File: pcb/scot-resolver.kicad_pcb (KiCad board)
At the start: 2 copper layers, 146 parts, among them IC1 AD8692ARMZ, IC10 AD2S1210, IC2 AD8397ARZ, IC3 AD8692ARMZ, IC4 TSR1, IC5 AD8692ARMZ, IC6 AD8692ARMZ, IC7 AD8692ARMZ, IC8 MCP2562, IC9 STM32F0xxKxTx, J1 Conn_01x02_Female, J2 Conn_01x02_Female, J3 Conn_01x02_Female, J4 Conn_01x03_Female, J5 Conn_01x03_Female, J6 Conn_01x03_Female, J7 CONN_01x03, P1 SWD, U1 MCP1703A-5002_SOT223, U2 LT1762, U3 MCP1703A-5002_SOT223, U4 MCP1703A-5002_SOT223, U5 MCP1703A-3302_SOT223, Y1 Crystal_GND24, Y2 Crystal

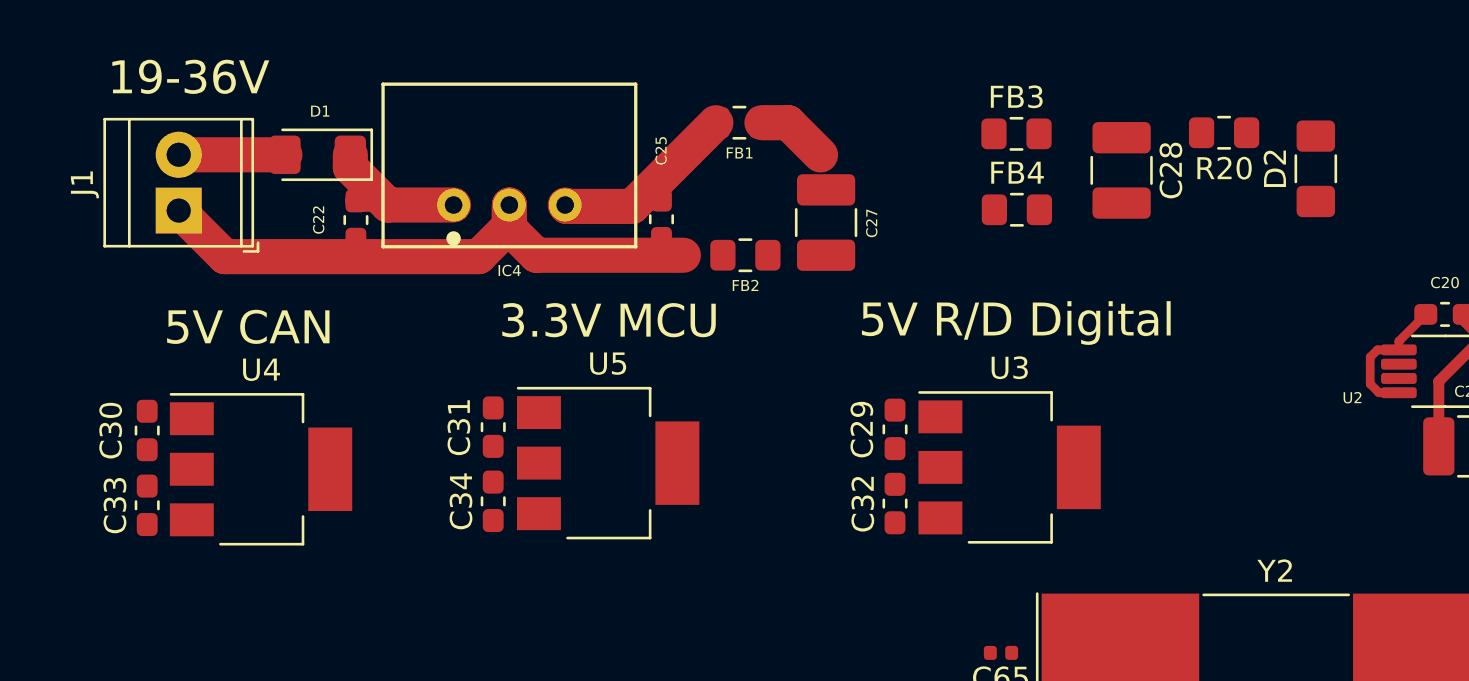
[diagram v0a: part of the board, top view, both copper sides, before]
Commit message: WIP.
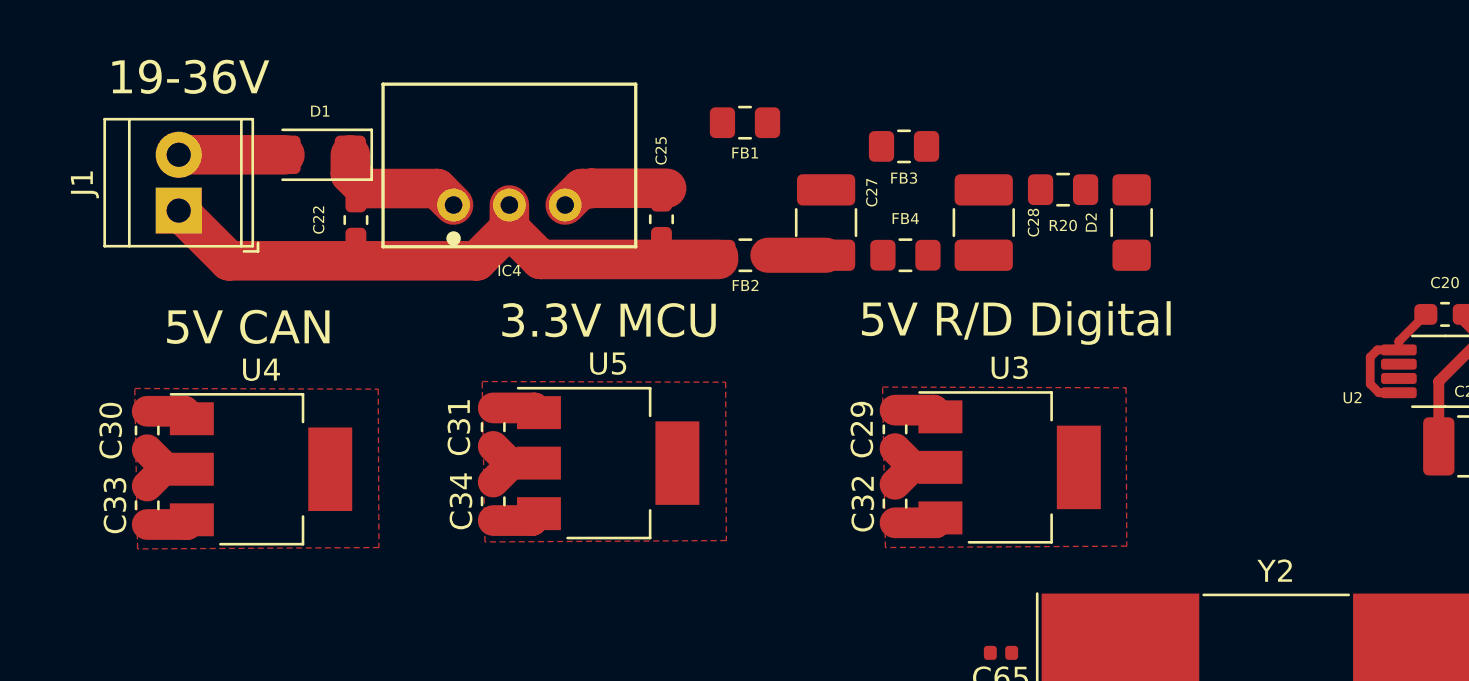
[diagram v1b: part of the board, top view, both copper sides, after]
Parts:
- moved D2 8.73 mm to (129.3, 60.9)
- moved R20 7.77 mm to (126.2, 59.4)
- moved C28 6.71 mm to (122.6, 60.9)
- moved FB4 5.48 mm to (119.0, 62.4)
- moved FB3 5.15 mm to (118.9, 57.5)
- moved FB1 0.25 mm to (111.7, 56.4)
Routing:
- net GND: track 0.00 -> 14.4 mm
- net +15V: track 0.00 -> 6.53 mm
- net Net-(C25-Pad1): track 8.46 -> 4.93 mm
- net AVCC: track 9.53 -> 6.26 mm
- net GNDA: track 80.4 -> 83.0 mm
- net /CAN TXRX/3.3V_MCU: track 0.00 -> 2.21 mm
- net /Microcontroller & Interface/5V_RESOLVER_DIGITAL: track 0.00 -> 2.16 mm
- net /CAN TXRX/5V_CAN: track 0.00 -> 2.12 mm
- net Net-(C22-Pad1): track 7.52 -> 6.16 mm
- net /Power Supplies/POWER_28V-: track 26.9 -> 28.1 mm
- added copper zone on F.Cu, net GND
